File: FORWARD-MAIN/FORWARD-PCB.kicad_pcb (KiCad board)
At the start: 4 copper layers, 96.3 x 67.5 mm, 41 parts, among them J1 USB_B_Micro, J2 Conn_01x03_Socket, J3 Conn_01x16_Socket, J4 Conn_01x08_Socket, U2 CP2102N-Axx-xQFN28, U5 ESP32-WROOM-32D

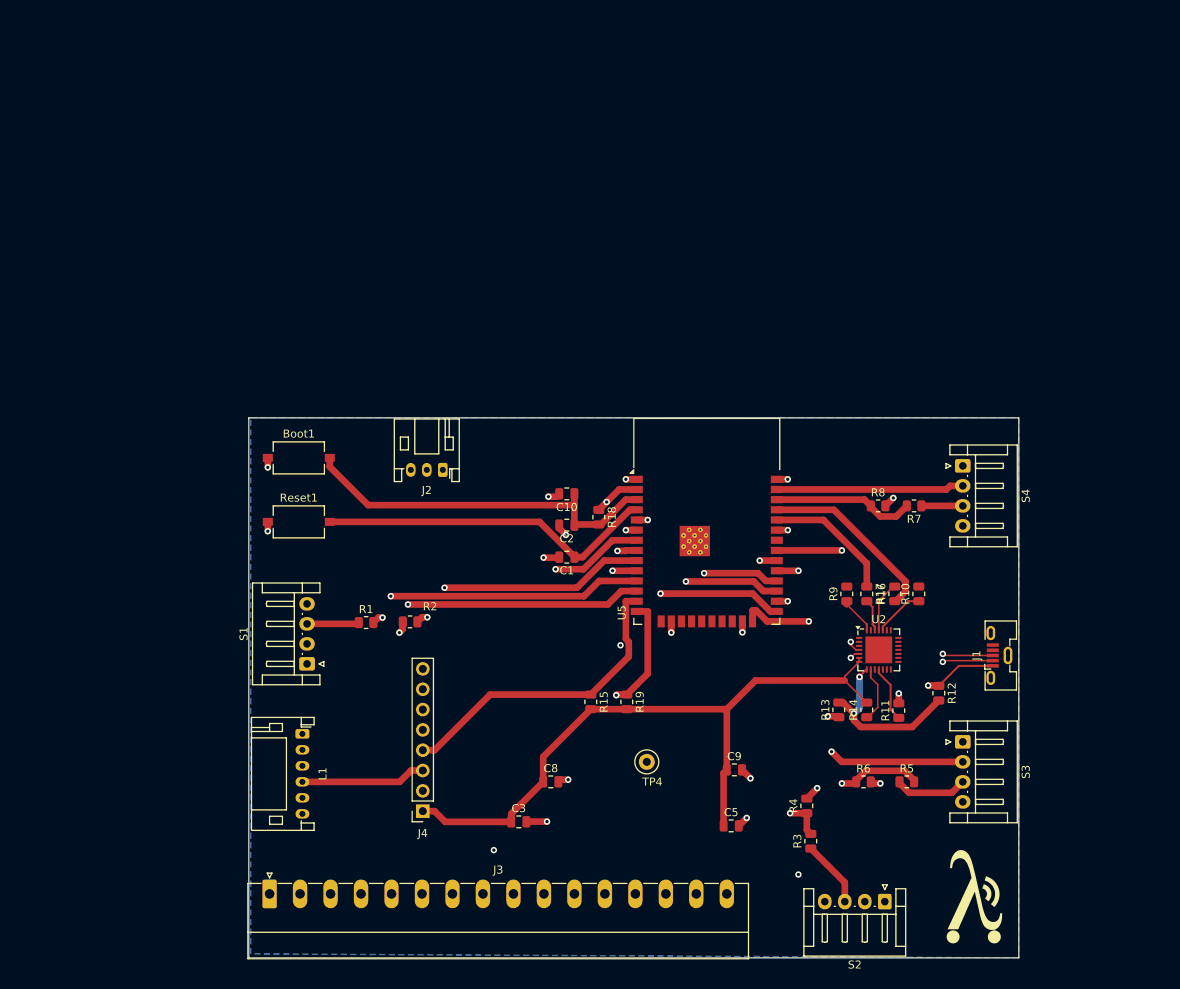
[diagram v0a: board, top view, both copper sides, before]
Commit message: itried
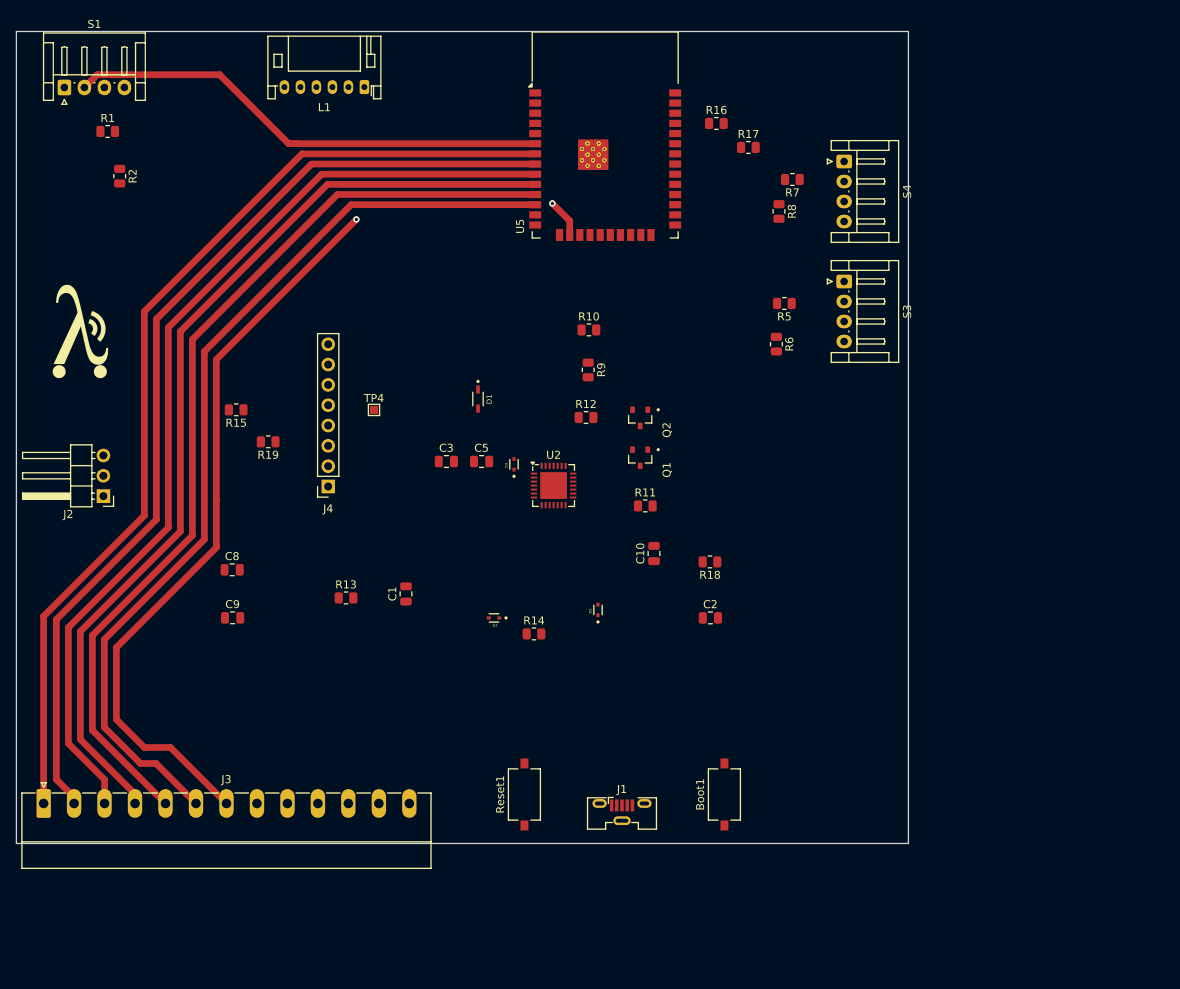
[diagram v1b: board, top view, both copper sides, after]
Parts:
- removed R3: 1k, Resistor_SMD:R_0805_2012Metric
- removed R4: 2k, Resistor_SMD:R_0805_2012Metric
- removed S2: Conn_01x04_Socket, Connector_JST:JST_EH_S4B-EH_1x04_P2.50mm_Horizontal
- added D1: BAT760-7, footprints:SOD2513X120N, F.Cu at (119.2, 94.4)
- added D2: LESD5D5.0CT1G, footprints:TVS_LESD5D5.0CT1G, F.Cu at (121.2, 121.8)
- added D3: LESD5D5.0CT1G, footprints:TVS_LESD5D5.0CT1G, F.Cu at (123.7, 102.6)
- added D5: LESD5D5.0CT1G, footprints:TVS_LESD5D5.0CT1G, F.Cu at (134.2, 120.8)
- added Q1: SS8050-G, footprints:TRANS_SS8050-G, F.Cu at (139.5, 101.8)
- added Q2: SS8050-G, footprints:TRANS_SS8050-G, F.Cu at (139.5, 96.8)
- J2: footprint Connector_JST:JST_PH_S3B-PH-K_1x03_P2.00mm_Horizontal -> Connector_PinHeader_2.54mm:PinHeader_1x03_P2.54mm_Horizontal
- J3: value Conn_01x16_Socket -> Conn_01x13_Socket; footprint Connector_Phoenix_MC:PhoenixContact_MC_1,5_16-G-3.81_1x16_P3.81mm_Horizontal -> Connector_Phoenix_MC:PhoenixContact_MC_1,5_13-G-3.81_1x13_P3.81mm_Horizontal
- TP4: footprint TestPoint:TestPoint_Loop_D2.50mm_Drill1.0mm_LowProfile -> TestPoint:TestPoint_Pad_1.0x1.0mm
- moved G*** 132.2 mm to (69.6, 85.1)
- moved L1 81.2 mm to (105.0, 55.5), turned to 180 degrees
- moved S1 78.2 mm to (67.5, 55.5), turned to 0 degrees
- moved R1 69.4 mm to (72.9, 61.0)
- moved Boot1 67.8 mm to (150.0, 143.9), turned to 90 degrees
- moved R2 66.5 mm to (74.4, 66.6), turned to -90 degrees
- moved C9 65.5 mm to (88.5, 121.8)
- moved R13 63.2 mm to (102.7, 119.3), turned to 0 degrees
- moved R16 62.9 mm to (149.0, 60.0), turned to 0 degrees
- moved R5 61.7 mm to (157.5, 82.5), turned to 180 degrees
- moved S3 59.4 mm to (165.0, 79.8)
- moved R17 57.7 mm to (153.0, 63.0), turned to 0 degrees
- moved R15 57.4 mm to (89.0, 95.8), turned to 180 degrees
- moved R12 56.0 mm to (132.7, 96.8), turned to 0 degrees
- moved R6 55.8 mm to (156.5, 87.6), turned to -90 degrees
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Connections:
- net /Wheels-IO16 renamed /Wheels-IO17-28
- net /Wheels-IO17 renamed /Wheels-IO5-29
- net /Wheels-IO18 renamed /Wheels-IO18-30
- net /Wheels-IO4 renamed /LIGHT-IO4-26
- net /Wheels-IO5 renamed /Wheels-IO16-27
- J3 pad 1: +5V -> /Haptics-IO25
- J3 pad 2: /Haptics-IO25 -> /Haptics-IO26
- J3 pad 3: /Haptics-IO26 -> /Haptics-IO27
- J3 pad 4: /Haptics-IO27 -> /Haptics-IO32
- J3 pad 5: /Haptics-IO32 -> /Haptics-IO33
- J3 pad 6: /Haptics-IO33 -> /Haptics-IO35
- J3 pad 7: /Haptics-IO35 -> /P0W-IO13-16
- J3 pad 8: /Wheels-IO0 -> /PHOTO-IO2-24
- R14 pad 1: Net-(U2-~{RST}) -> /RST
- U2 pad 9: Net-(U2-~{RST}) -> /RST
- U5 pad 10: /Haptics-IO25 -> /Haptics-IO32
- U5 pad 11: /Haptics-IO26 -> /Haptics-IO33
- U5 pad 12: /Haptics-IO27 -> /Haptics-IO35
- U5 pad 16: /P0W -> /P0W-IO13-16
- U5 pad 23: /ECHO_2 -> /ECHO_1
- U5 pad 24: /TRIG_2 -> /PHOTO-IO2-24
- U5 pad 25: /Wheels-IO0 -> /IO0
- U5 pad 4: /RST -> unconnected-(U5-SENSOR_VP-Pad4)
- U5 pad 5: /ECHO_1 -> unconnected-(U5-SENSOR_VN-Pad5)
- U5 pad 7: /Haptics-IO35 -> /Haptics-IO25
- U5 pad 8: /Haptics-IO32 -> /Haptics-IO26
- U5 pad 9: /Haptics-IO33 -> /Haptics-IO27
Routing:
- net +5V: track 195.8 -> 0.00 mm
- net +3.3V: track 163.0 -> 0.00 mm, vias 1 -> 0
- net /P0W-IO13-16: track 0.00 -> 123.2 mm, vias 0 -> 2
- net /Wheels-IO16-27: track 74.9 -> 0.00 mm, vias 2 -> 0
- net /Wheels-IO0: track 62.4 -> 0.00 mm, vias 1 -> 0
- net /LIGHT-IO4-26: track 61.2 -> 0.00 mm, vias 2 -> 0
- net /Haptics-IO35: track 57.6 -> 116.5 mm, vias 1 -> 0
- net /SCL: track 57.9 -> 0.00 mm, vias 1 -> 0
- net /Wheels-IO18-30: track 57.7 -> 0.00 mm, vias 1 -> 0
- net /Wheels-IO17-28: track 56.7 -> 0.00 mm, vias 1 -> 0
- net /SDA: track 56.6 -> 0.00 mm
- net /Wheels-IO5-29: track 54.7 -> 0.00 mm, vias 1 -> 0
- net /Haptics-IO33: track 64.9 -> 117.3 mm, vias 1 -> 0
- net /Haptics-IO27: track 67.9 -> 120.3 mm, vias 1 -> 0
- net /Haptics-IO25: track 72.0 -> 123.7 mm, vias 2 -> 0
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- added copper zone on In1.Cu, net GND
- removed copper zone on B.Cu, net GND
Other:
- board size 96.3 x 67.5 mm -> 111.5 x 101.5 mm

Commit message: a good iteration!
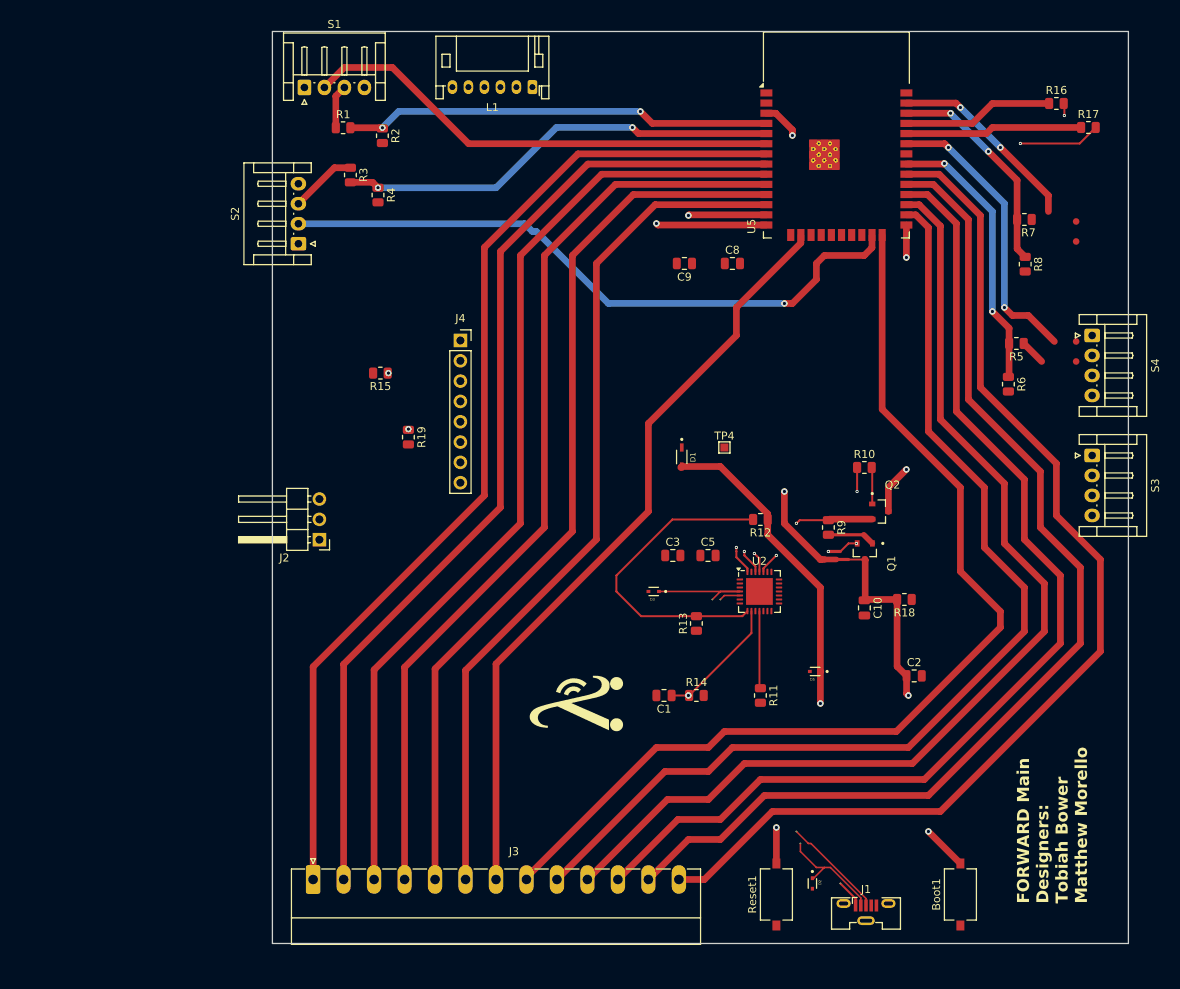
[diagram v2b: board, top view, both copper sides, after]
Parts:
- added R3: 1k, Resistor_SMD:R_0805_2012Metric, F.Cu at (103.2, 66.4)
- added R4: 2k, Resistor_SMD:R_0805_2012Metric, F.Cu at (106.7, 68.9)
- added S2: Conn_01x04_Socket, Connector_JST:JST_EH_S4B-EH_1x04_P2.50mm_Horizontal, F.Cu at (96.8, 75.0)
- moved G*** 77.3 mm to (130.6, 132.4), turned to 90 degrees
- moved C8 73.3 mm to (151.0, 77.5)
- moved C9 71.8 mm to (145.0, 77.5), turned to 180 degrees
- moved D2 51.8 mm to (161.0, 155.0), turned to -90 degrees
- moved TP4 44.1 mm to (150.0, 100.5)
- moved R13 43.9 mm to (146.5, 122.5), turned to 90 degrees
- moved R16 42.6 mm to (191.5, 57.5)
- moved R17 42.6 mm to (195.5, 60.5)
- moved R10 38.5 mm to (167.5, 103.0)
- moved S3 37.9 mm to (196.0, 101.5)
- moved S4 37.9 mm to (196.0, 86.5)
- moved R9 35.9 mm to (163.0, 110.5)
- moved J3 35.0 mm to (98.6, 154.5)
- moved C1 34.7 mm to (142.4, 131.5), turned to 180 degrees
- moved Reset1 33.9 mm to (156.5, 156.4)
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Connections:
- net /Haptics-IO25 renamed /Haptics-IN1
- net /Haptics-IO26 renamed /Haptics-IN2
- net /Haptics-IO27 renamed /Haptics-IN3
- net /Haptics-IO32 renamed /Haptics-IN4
- net /Haptics-IO33 renamed /Haptics-ENA_PWM
- net /Haptics-IO35 renamed /Haptics-ENB_PWM
- net /Wheels-IO18-30 renamed /IO18-30
- J3 pad 10: /Wheels-IO16-27 -> /Wheels-RPWM
- J3 pad 11: /Wheels-IO17-28 -> /Wheels_LPWM
- J3 pad 12: /Wheels-IO5-29 -> /IO16-27
- U5 pad 23: /ECHO_1 -> /TRIG_2
- U5 pad 27: /Wheels-IO17-28 -> /Wheels-RPWM
- U5 pad 28: /Wheels-IO5-29 -> /Wheels_LPWM
- U5 pad 29: /Wheels-IO16-27 -> /IO16-27
- U5 pad 4: unconnected-(U5-SENSOR_VP-Pad4) -> /ECHO_1
- U5 pad 5: unconnected-(U5-SENSOR_VN-Pad5) -> /ECHO_2
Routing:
- net /IO18-30: track 0.00 -> 136.6 mm
- net /IO16-27: track 0.00 -> 134.6 mm
- net /Wheels_LPWM: track 0.00 -> 133.2 mm
- net /Wheels-RPWM: track 0.00 -> 131.4 mm
- net /LIGHT-IO4-26: track 0.00 -> 130.1 mm
- net /PHOTO-IO2-24: track 0.00 -> 127.6 mm
- net /SCL: track 0.00 -> 117.0 mm, vias 0 -> 2
- net /EN: track 0.00 -> 114.6 mm, vias 0 -> 4
- net /SDA: track 0.00 -> 96.3 mm, vias 0 -> 2
- net /TXD: track 0.00 -> 83.6 mm, vias 0 -> 2
- net /TRIG_2: track 0.00 -> 81.5 mm, vias 0 -> 1
- net /RXD: track 0.00 -> 80.5 mm, vias 0 -> 2
- net /VBUS: track 0.00 -> 66.9 mm, vias 0 -> 2
- net /USB_DP: track 0.00 -> 60.3 mm, vias 0 -> 2
- net /ECHO_2: track 0.00 -> 55.7 mm, vias 0 -> 2
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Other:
- board size 111.5 x 101.5 mm -> 107 x 114 mm
- board text added: "FORWARD Main Designers: Tobiah Bower Matthew Morello"
